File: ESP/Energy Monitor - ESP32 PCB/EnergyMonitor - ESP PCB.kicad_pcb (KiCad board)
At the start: 4 copper layers, 9 parts, among them J10 Conn_01x04, J11 Conn_01x05, J12 Conn_01x05, J8 Conn_01x04, J9 Conn_01x04

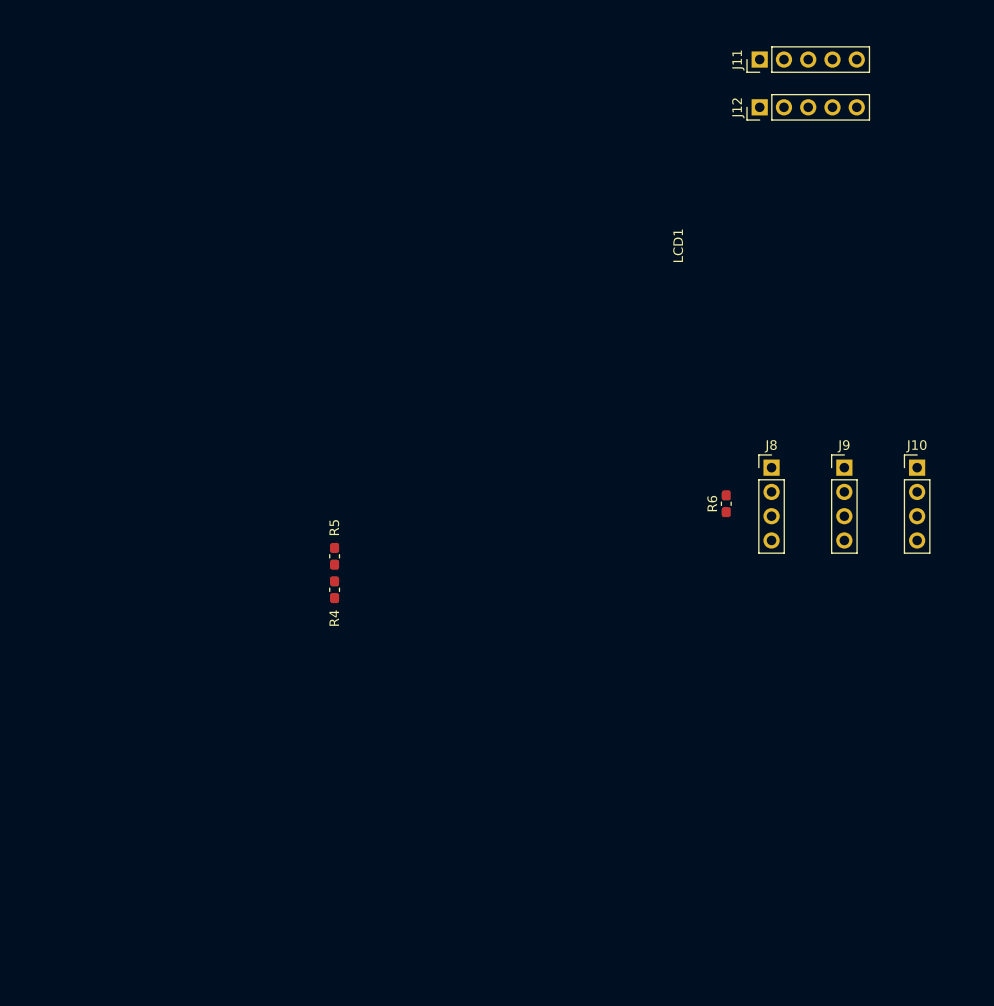
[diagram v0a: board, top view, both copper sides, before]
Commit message: Projects Projects Projects Projects.
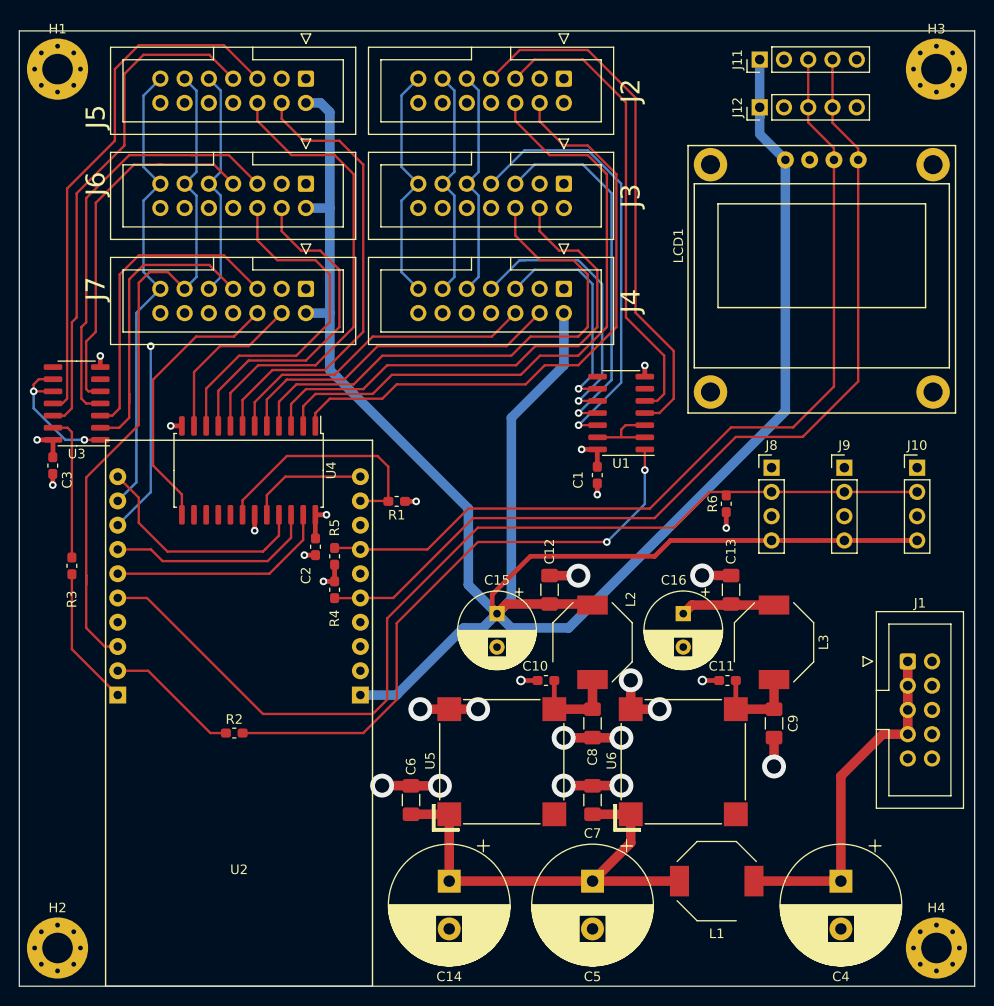
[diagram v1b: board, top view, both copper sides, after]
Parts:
- added C1: 0.1 uF, Capacitor_SMD:C_0603_1608Metric_Pad1.05x0.95mm_HandSolder, F.Cu at (100.5, 86.5)
- added C10: 0.1 uF, Capacitor_SMD:C_0603_1608Metric_Pad1.05x0.95mm_HandSolder, F.Cu at (95.1, 108.0)
- added C11: 0.1 uF, Capacitor_SMD:C_0603_1608Metric_Pad1.05x0.95mm_HandSolder, F.Cu at (114.1, 108.0)
- added C12: 22 uF, Capacitor_SMD:C_1206_3216Metric_Pad1.42x1.75mm_HandSolder, F.Cu at (95.5, 98.5)
- added C13: 22 uF, Capacitor_SMD:C_1206_3216Metric_Pad1.42x1.75mm_HandSolder, F.Cu at (114.5, 98.5)
- added C14: CP1, Capacitor_THT:CP_Radial_D12.5mm_P5.00mm, F.Cu at (85.0, 129.0)
- added C15: CP1, Capacitor_THT:CP_Radial_D8.0mm_P3.50mm, F.Cu at (90.0, 101.0)
- added C16: CP1, Capacitor_THT:CP_Radial_D8.0mm_P3.50mm, F.Cu at (109.5, 101.0)
- added C2: 0.1 uF, Capacitor_SMD:C_0603_1608Metric_Pad1.05x0.95mm_HandSolder, F.Cu at (71.0, 94.0)
- added C3: 0.1 uF, Capacitor_SMD:C_0603_1608Metric_Pad1.05x0.95mm_HandSolder, F.Cu at (43.5, 85.5)
- added C4: CP1, Capacitor_THT:CP_Radial_D12.5mm_P5.00mm, F.Cu at (126.0, 129.0)
- added C5: CP1, Capacitor_THT:CP_Radial_D12.5mm_P5.00mm, F.Cu at (100.0, 129.0)
- added C6: 10 uF, 35V, Capacitor_SMD:C_1206_3216Metric_Pad1.42x1.75mm_HandSolder, F.Cu at (81.0, 120.5)
- added C7: 10 uF, 35V, Capacitor_SMD:C_1206_3216Metric_Pad1.42x1.75mm_HandSolder, F.Cu at (100.0, 120.5)
- added C8: 22 uF, Capacitor_SMD:C_1206_3216Metric_Pad1.42x1.75mm_HandSolder, F.Cu at (100.0, 112.5)
- added C9: 22 uF, Capacitor_SMD:C_1206_3216Metric_Pad1.42x1.75mm_HandSolder, F.Cu at (119.0, 112.5)
- added H1: MountingHole, MountingHole:MountingHole_3.2mm_M3_Pad_Via, F.Cu at (44.0, 44.0)
- added H2: MountingHole, MountingHole:MountingHole_3.2mm_M3_Pad_Via, F.Cu at (44.0, 136.0)
- added H3: MountingHole, MountingHole:MountingHole_3.2mm_M3_Pad_Via, F.Cu at (136.0, 44.0)
- added H4: MountingHole, MountingHole:MountingHole_3.2mm_M3_Pad_Via, F.Cu at (136.0, 136.0)
- added J1: Conn_02x05_Odd_Even, Connector_IDC:IDC-Header_2x05_P2.54mm_Vertical, F.Cu at (133.0, 106.0)
- added J2: Conn_02x07_Odd_Even, Connector_IDC:IDC-Header_2x07_P2.54mm_Vertical, F.Cu at (97.0, 45.0)
- added J3: Conn_02x07_Odd_Even, Connector_IDC:IDC-Header_2x07_P2.54mm_Vertical, F.Cu at (97.0, 56.0)
- added J4: Conn_02x07_Odd_Even, Connector_IDC:IDC-Header_2x07_P2.54mm_Vertical, F.Cu at (97.0, 67.0)
- added J5: Conn_02x07_Odd_Even, Connector_IDC:IDC-Header_2x07_P2.54mm_Vertical, F.Cu at (70.0, 45.0)
- added J6: Conn_02x07_Odd_Even, Connector_IDC:IDC-Header_2x07_P2.54mm_Vertical, F.Cu at (70.0, 56.0)
- added J7: Conn_02x07_Odd_Even, Connector_IDC:IDC-Header_2x07_P2.54mm_Vertical, F.Cu at (70.0, 67.0)
- added L1: 47 uH, Inductor_SMD:L_Bourns-SRU8028_8.0x8.0mm, F.Cu at (113.0, 129.0)
- added L2: 47 uH, Inductor_SMD:L_Bourns-SRU8028_8.0x8.0mm, F.Cu at (100.0, 104.0)
- added L3: 47 uH, Inductor_SMD:L_Bourns-SRU8028_8.0x8.0mm, F.Cu at (119.0, 104.0)
- added R1: 10K, Resistor_SMD:R_0603_1608Metric_Pad1.05x0.95mm_HandSolder, F.Cu at (79.5, 89.2)
- added R2: 330R, Resistor_SMD:R_0603_1608Metric_Pad1.05x0.95mm_HandSolder, F.Cu at (62.5, 113.5)
- added R3: 330R, Resistor_SMD:R_0603_1608Metric_Pad1.05x0.95mm_HandSolder, F.Cu at (45.5, 96.0)
- added U1: 4072, Package_SO:SOIC-14_3.9x8.7mm_P1.27mm, F.Cu at (103.0, 80.0)
- added U2: ESP32-POE Module, Energy Monitor - ESP32 PCB:ESP32-POE, F.Cu at (63.0, 140.0)
- added U3: 4072, Package_SO:SOIC-14_3.9x8.7mm_P1.27mm, F.Cu at (46.0, 79.0)
- added U4: 4072, Package_SO:SOIC-24W_7.5x15.4mm_P1.27mm, F.Cu at (64.0, 86.0)
- added U5: VXO7805-500-M, custom:VXO78x-500-M, F.Cu at (90.5, 116.5)
- added U6: VXO7803-500-M, custom:VXO78x-500-M, F.Cu at (109.5, 116.5)
- LCD1: value 0.96 -> 0.96"-SSD1306-DISP-I2C
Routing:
- net +5V: track 0.00 -> 285.5 mm
- net /ESP1/MISO: track 0.00 -> 127.1 mm
- net /ESP1/MOSI: track 0.00 -> 115.5 mm, vias 0 -> 1
- net GND: track 0.00 -> 104.8 mm, vias 0 -> 22
- net Net-(J10-Pad2): track 0.00 -> 103.8 mm
- net /ESP1/SCLK: track 0.00 -> 103.4 mm
- net Net-(J11-Pad4): track 0.00 -> 99.0 mm
- net Net-(J11-Pad3): track 0.00 -> 94.7 mm
- net /ESP1/~{CS_2}: track 0.00 -> 67.1 mm
- net /ESP1/~{CS_1}: track 0.00 -> 64.8 mm
- net Net-(R2-Pad2): track 0.00 -> 62.4 mm, vias 0 -> 2
- net /ESP1/~{CS_4}: track 0.00 -> 55.7 mm
- net /ESP1/IRQ_7: track 0.00 -> 55.7 mm
- net /ESP1/IRQ_2: track 0.00 -> 55.2 mm
- net /ESP1/~{CS_3}: track 0.00 -> 53.8 mm
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- added copper zone on In2.Cu, net +3V3
- added copper zone on In1.Cu, net GND
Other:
- board outline added: 100 x 100 mm
- net class Default removed
